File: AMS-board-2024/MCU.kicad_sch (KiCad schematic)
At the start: 127 parts, among them Q105 2N7002K-AU, Q106 2N7002K-AU, Q107 2N7002K-AU, Q108 2N7002K-AU, SW1 DS04-254-01BK-SMT, SW2 PTS636-SL43-SMTR, U10 TCAN1042DQ1, U11 LTC6820, U12 R7FA4M1AB3CFM#AA0, U13 BD5230G-2MTR, U14 TMP101-Q1, U15 NV24C16SNVLT3G, U16 TPS2561QDRCRQ1, U17 TPS2561QDRCRQ1, U9 ADUM3160, Y1 ABM8W

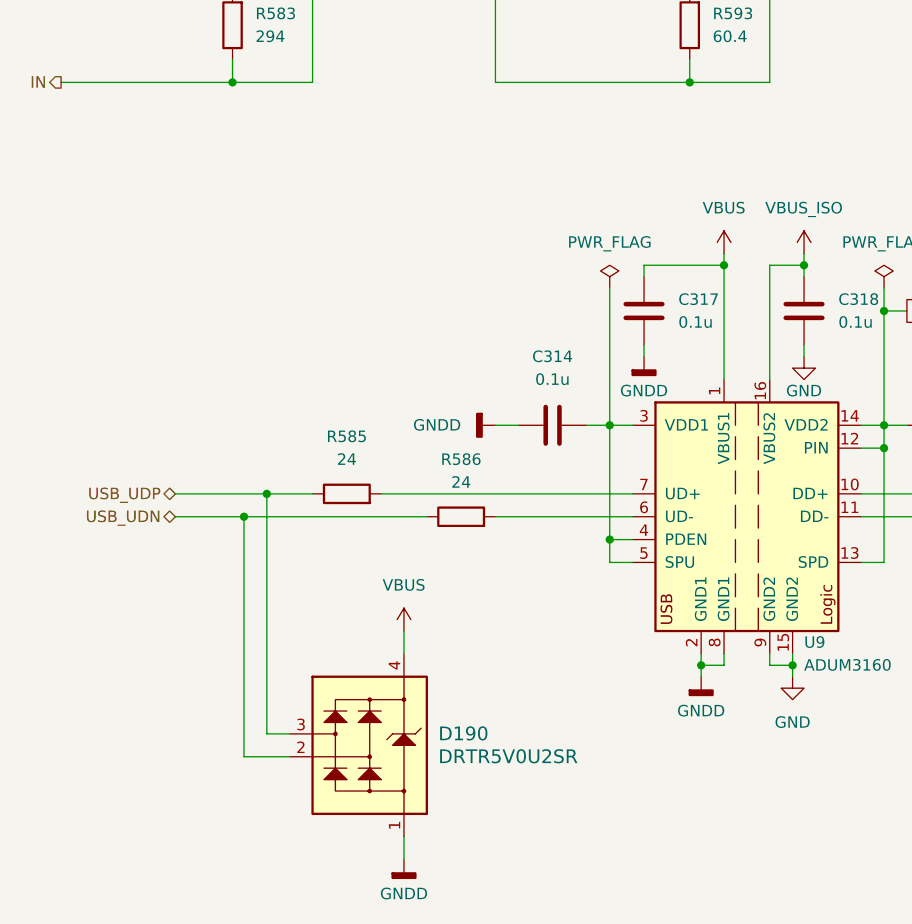
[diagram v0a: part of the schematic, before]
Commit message: 階層シート内の電源シンボル修正
階層シート内で電源シンボルをなるべく使わないようにする
修正途中
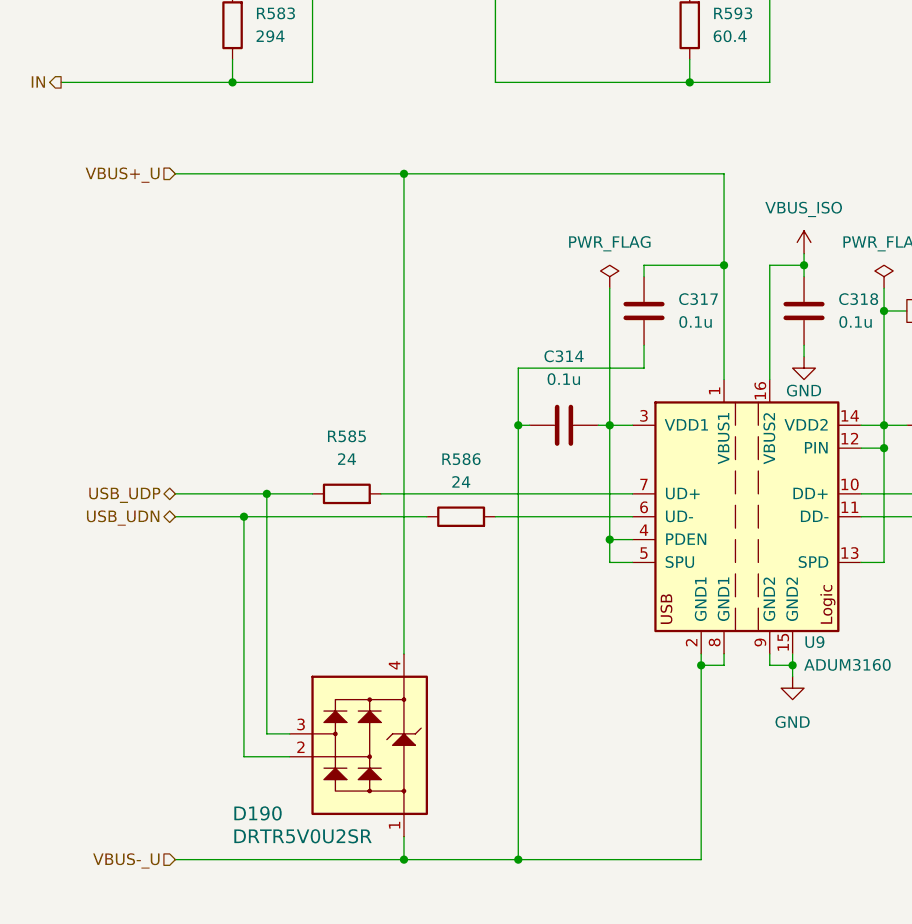
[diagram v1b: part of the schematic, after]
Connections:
- net VBUS: no longer C317.2, D190.4, U9.1 (VBUS1)
- net GNDD renamed VBUS-_U
- new net VBUS+_U: C317.2, D190.4, U9.1 (VBUS1)
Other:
- moved on the sheet: C314
